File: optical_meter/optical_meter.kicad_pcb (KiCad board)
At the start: 4 copper layers, 74 x 72 mm, 46 parts, among them J1 Conn_02x04, J2 SFP+, J3 Conn_01x02_Pin, U2 FIN1002M5X, U3 FIN1001M5X, U5 Pico

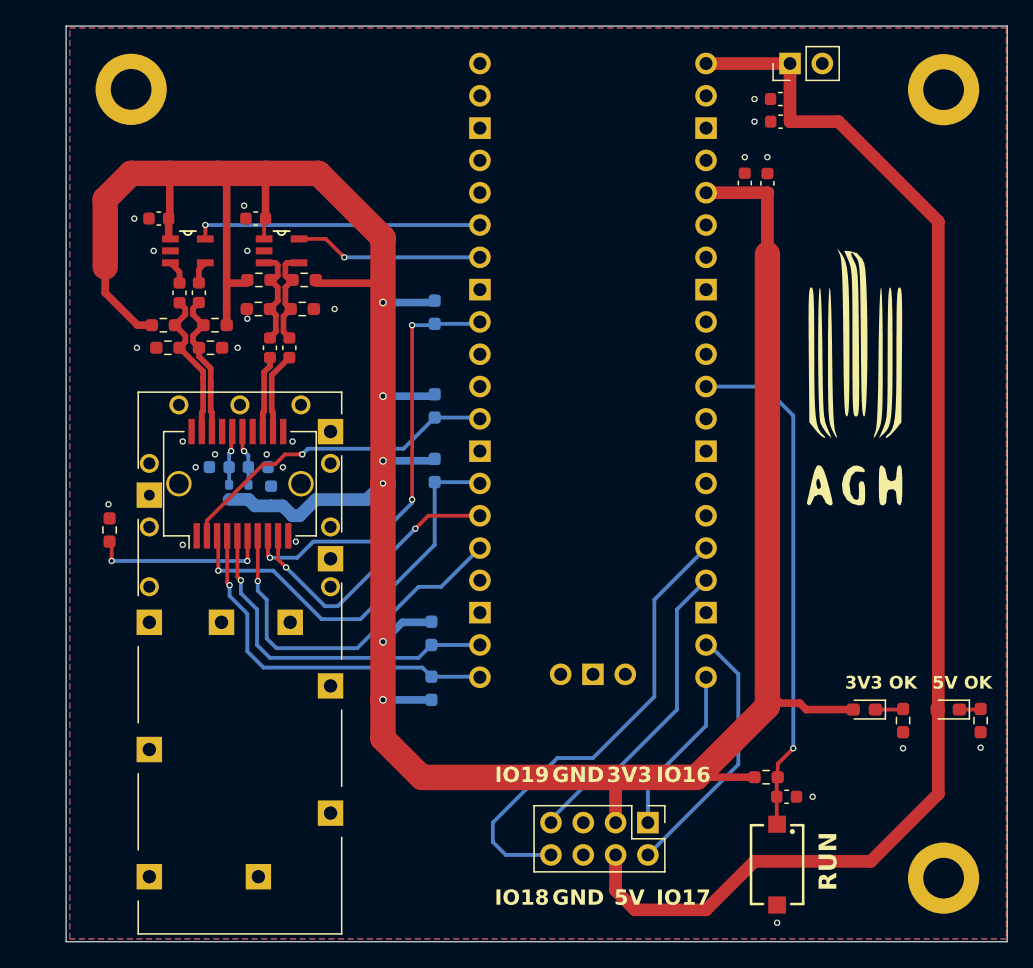
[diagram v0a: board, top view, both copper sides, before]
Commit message: changing the layout (in progress)
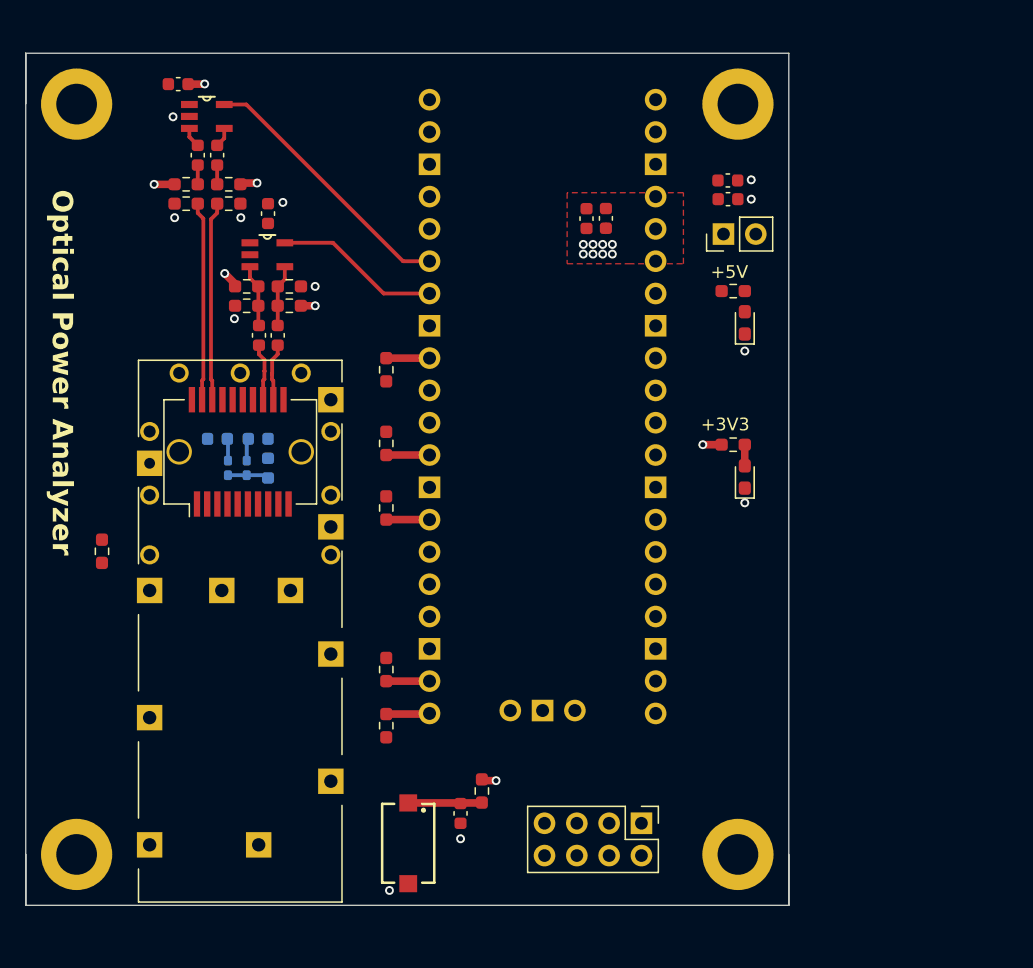
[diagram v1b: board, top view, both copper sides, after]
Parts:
- removed G***: LOGO, AGH_LOGO:agh_logo
- removed the H4 at (242.7, 87.2)
- removed H5: ~, MountingHole:MountingHole_3.2mm_M3_DIN965_Pad
- removed the H6 at (178.8, 25.1)
- added H4: ~, MountingHole:MountingHole_3.2mm_M3_DIN965_Pad, F.Cu at (226.5, 85.3)
- added H4: ~, MountingHole:MountingHole_3.2mm_M3_DIN965_Pad, F.Cu at (174.5, 85.3)
- added H6: ~, MountingHole:MountingHole_3.2mm_M3_DIN965_Pad, F.Cu at (174.5, 26.3)
- added H6: ~, MountingHole:MountingHole_3.2mm_M3_DIN965_Pad, F.Cu at (226.5, 26.3)
- C10, C27: value 2u2 -> 4u7
- R11, R20, R6, R7, R8: moved to F.Cu
- R2: value 1k -> 680R
- moved R1 39.0 mm to (226.2, 41.0), turned to 0 degrees
- moved D1 34.4 mm to (227.1, 43.5), turned to 90 degrees
- moved S2 29.1 mm to (200.6, 84.4)
- moved C25 25.7 mm to (204.7, 82.1), turned to 90 degrees
- moved R2 25.5 mm to (226.2, 53.1), turned to 0 degrees
- moved R10 22.4 mm to (206.4, 80.3), turned to -90 degrees
- moved D2 20.6 mm to (227.1, 55.6), turned to 90 degrees
- moved J3 14.4 mm to (225.4, 36.5)
- moved C27 13.0 mm to (216.2, 35.3)
- moved C28 12.8 mm to (214.6, 35.3)
- moved R17 11.4 mm to (186.5, 34.1)
- moved R19 11.4 mm to (183.1, 34.1)
- moved R18 11.2 mm to (183.1, 32.6)
- moved R16 11.1 mm to (186.5, 32.6)
- moved C29 10.9 mm to (184.1, 30.3)
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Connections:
- D1 pad 1: Net-(D1-K) -> GND
- D1 pad 2: +5V -> Net-(D1-A)
- D2 pad 1: Net-(D2-K) -> GND
- D2 pad 2: +3V3 -> Net-(D2-A)
- J1 pad 4: +5V -> +3V3
- R1 pad 1: Net-(D1-K) -> +5V
- R1 pad 2: GND -> Net-(D1-A)
- R2 pad 1: Net-(D2-K) -> +3V3
- R2 pad 2: GND -> Net-(D2-A)
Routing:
- net +3V3: track 233.3 -> 12.4 mm, vias 6 -> 15
- net +5V: track 103.7 -> 0.00 mm
- net /GPIO19: track 37.4 -> 0.00 mm
- net /RUN: track 40.5 -> 5.65 mm, vias 1 -> 0
- net /RX_LOS: track 34.2 -> 3.41 mm, vias 3 -> 0
- net /TX_DISABLE: track 32.3 -> 3.40 mm, vias 1 -> 0
- net /RS0: track 28.7 -> 0.00 mm, vias 1 -> 0
- net /SDA: track 28.9 -> 3.42 mm, vias 1 -> 0
- net /GPIO18: track 24.8 -> 0.00 mm
- net /SCL: track 27.6 -> 3.40 mm, vias 1 -> 0
- net /TX_FAULT: track 26.3 -> 3.40 mm, vias 1 -> 0
- net /RS1: track 22.2 -> 0.00 mm, vias 2 -> 0
- net /GPIO17: track 20.7 -> 0.00 mm
- net Net-(J2-MOD_ABS): track 14.2 -> 0.00 mm, vias 2 -> 0
- net /GPIO16: track 13.3 -> 0.00 mm
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- added copper zone on F.Cu, net +3V3
- added copper zone on In2.Cu, net +3V3
- added copper zone on In2.Cu, net +5V
- removed copper zone on B.Cu, net GND
- removed copper zone on F.Cu, net GND
- removed copper zone on In2.Cu, net GND
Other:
- board size 74 x 72 mm -> 60 x 67 mm
- board text added: "+3V3"
- board text added: "+5V"
- board text added: "Optical Power Analyzer"
- board text removed: "3V3"
- board text removed: "3V3 OK"
- board text removed: "5V"
- board text removed: "5V OK"
- board text removed: "GND"
- board text removed: "IO16"
- board text removed: "IO17"
- board text removed: "IO18"
- board text removed: "IO19"
- board text removed: "PCB by Filip Kulka"
- board text removed: "RUN"
